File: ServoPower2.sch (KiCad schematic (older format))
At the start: 16 parts, among them J1 Conn_01x03, J10 Conn_01x03, J11 Conn_01x03, J12 Conn_01x03, J13 Conn_01x02, J14 Conn_01x02, J15 Conn_01x02, J2 Conn_01x03, J3 Conn_01x03, J4 Conn_01x03, J5 Conn_01x03, J6 Conn_01x03, J7 Conn_01x03, J8 Conn_01x03, J9 Conn_01x03, U1 Teensy4.0

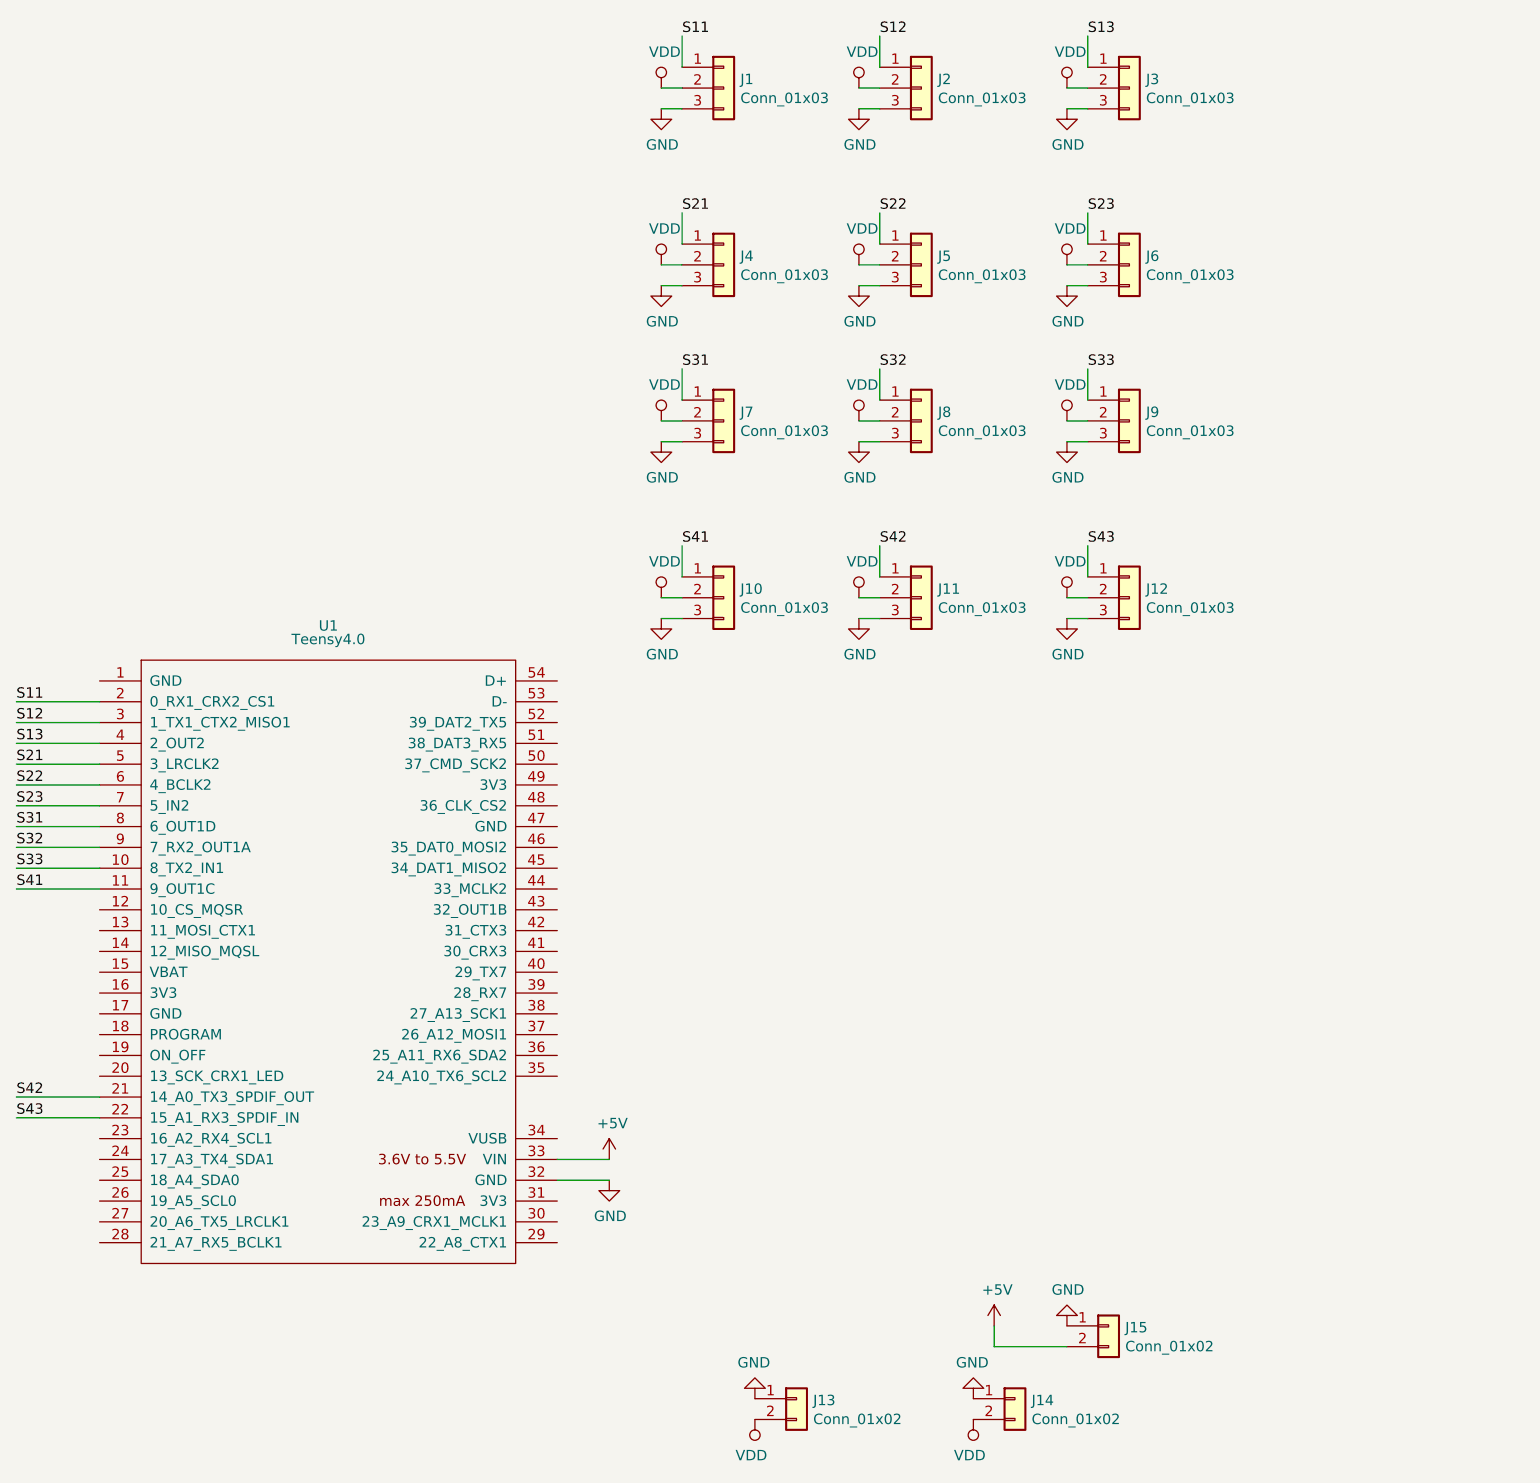
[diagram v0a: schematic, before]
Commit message: clean up
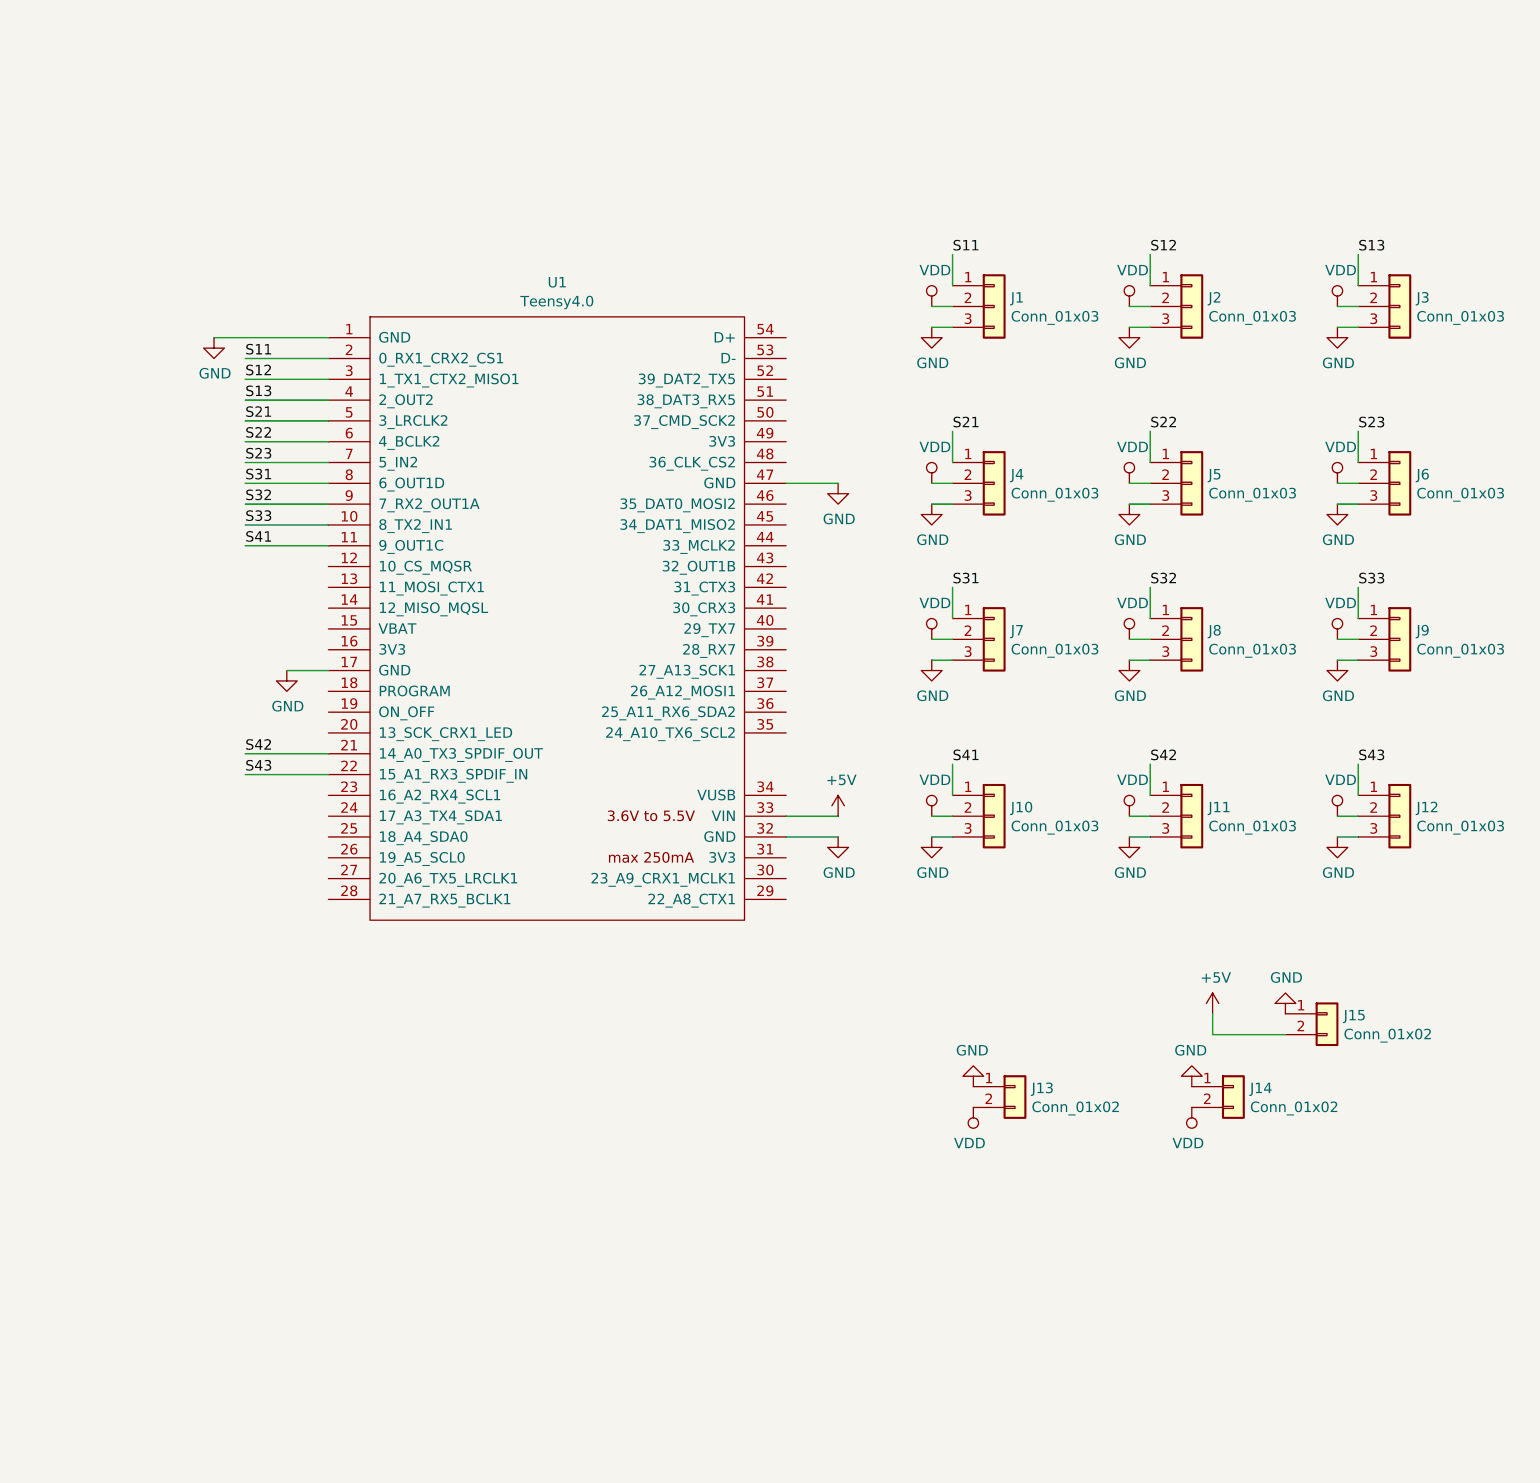
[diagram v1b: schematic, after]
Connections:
- net GND: now also U1.1 (GND), U1.17 (GND), U1.47 (GND)
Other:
- moved on the sheet: J1, J10, J11, J12, J13, J14, J15, J2, J3, J4, J5, J6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
